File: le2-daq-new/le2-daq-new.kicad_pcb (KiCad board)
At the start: 2 copper layers, 62 x 105.9 mm, 9 parts, among them J1 RELAY-CONN, J2 CAP-CONN, J3 TC-CONN, J4 HX_CON, J5 Conn_01x02_Male, SW1 SW_Push, U1 ESP32-DEVKITC-32D

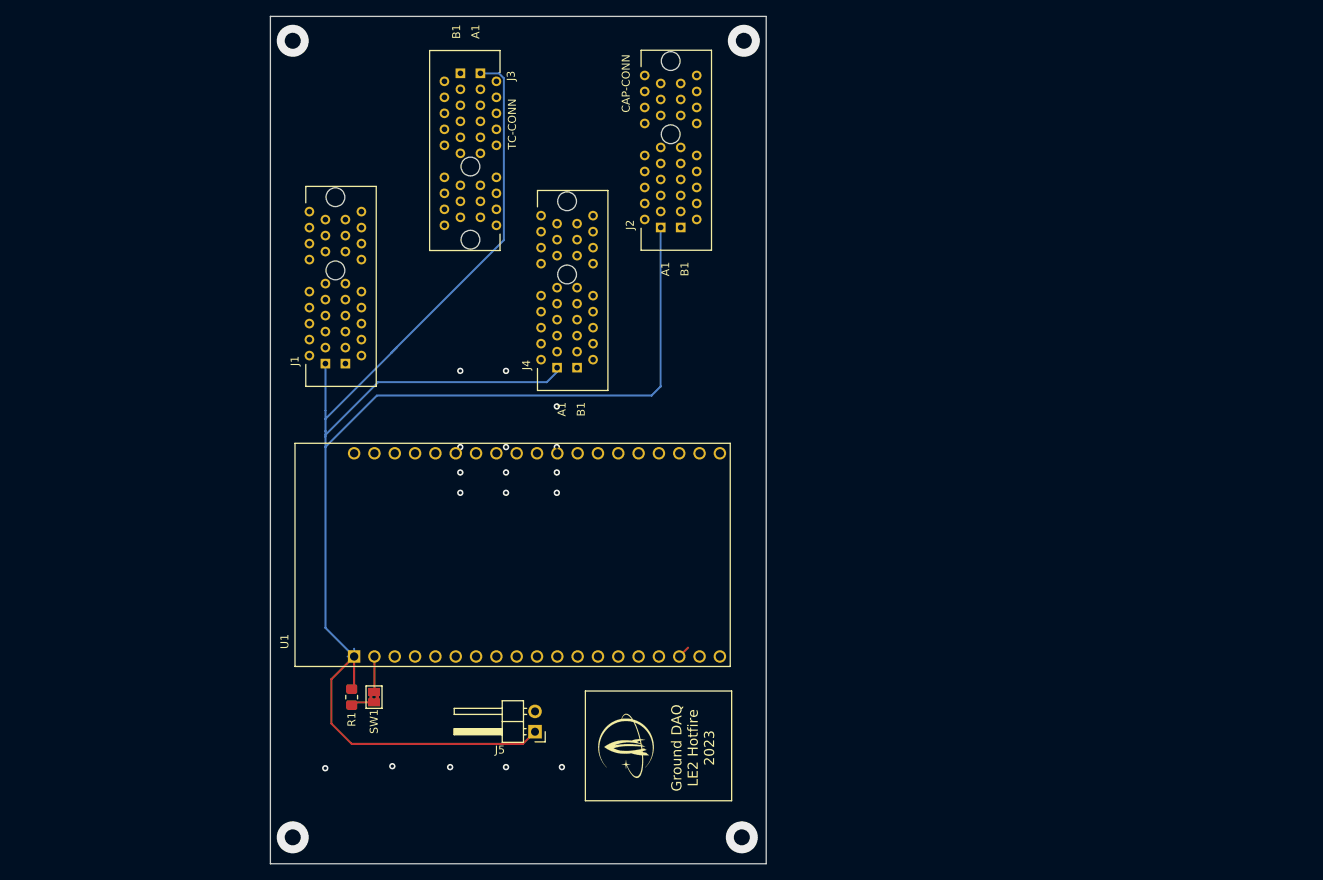
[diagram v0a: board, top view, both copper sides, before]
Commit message: CORE PCB DONE
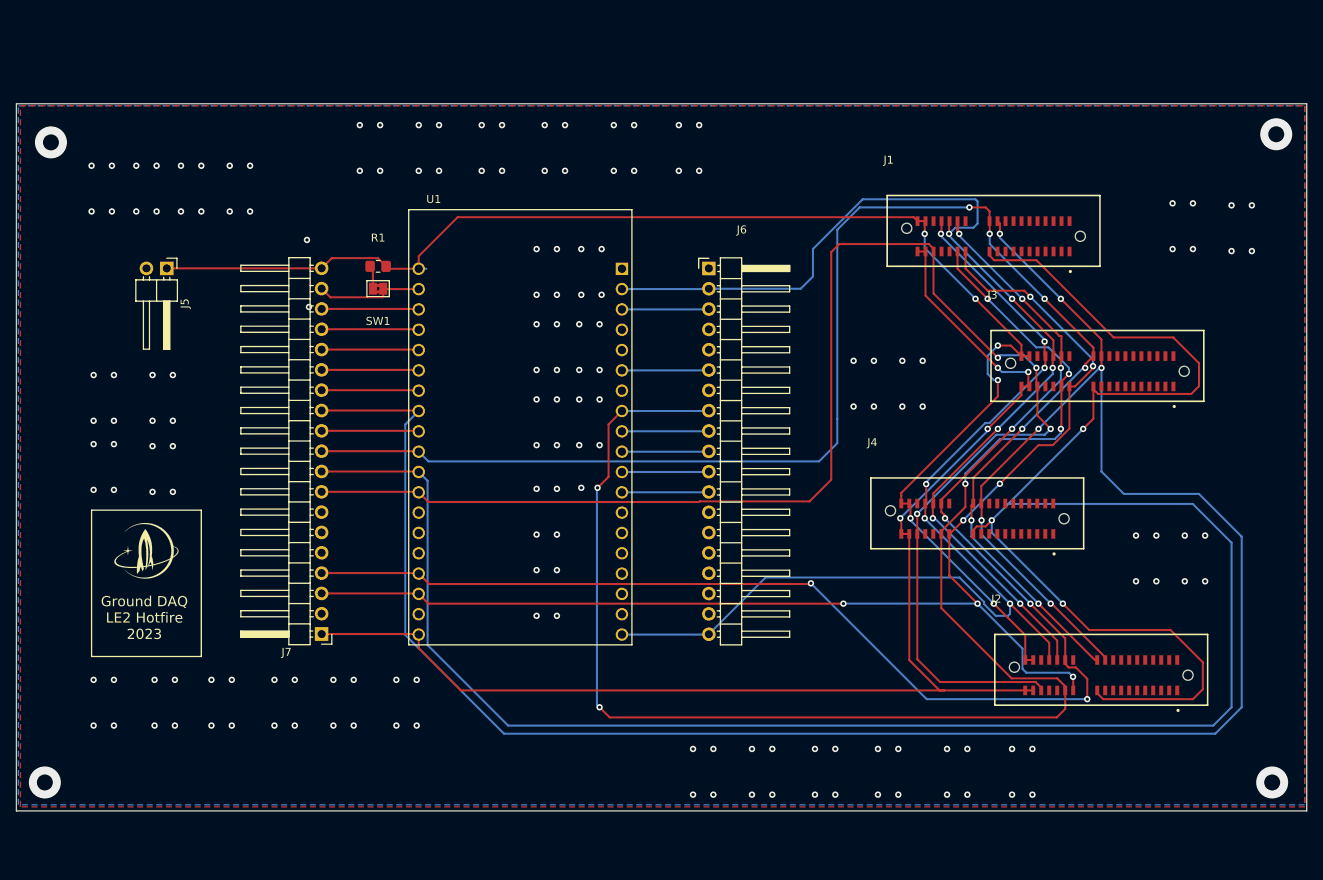
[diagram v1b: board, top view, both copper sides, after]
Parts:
- added J6: TEST-POINT, Connector_PinHeader_2.54mm:PinHeader_1x19_P2.54mm_Horizontal, F.Cu at (140.7, 78.2)
- added J7: TEST-POINT, Connector_PinHeader_2.54mm:PinHeader_1x19_P2.54mm_Horizontal, F.Cu at (92.3, 123.9)
- J1: value RELAY-CONN -> PCIE_CONN; footprint PCIE_1x_Socket:AMPHENOL_10018784-10210TLF -> PCIE-LP-01-01-F-DV-A-TR:SAMTEC_PCIE-LP-01-01-F-DV-A-TR
- J2: value CAP-CONN -> PCIE_CONN; footprint PCIE_1x_Socket:AMPHENOL_10018784-10210TLF -> PCIE-LP-01-01-F-DV-A-TR:SAMTEC_PCIE-LP-01-01-F-DV-A-TR
- J3: value TC-CONN -> PCIE_CONN; footprint PCIE_1x_Socket:AMPHENOL_10018784-10210TLF -> PCIE-LP-01-01-F-DV-A-TR:SAMTEC_PCIE-LP-01-01-F-DV-A-TR
- J4: value HX_CON -> PCIE_CONN; footprint PCIE_1x_Socket:AMPHENOL_10018784-10210TLF -> PCIE-LP-01-01-F-DV-A-TR:SAMTEC_PCIE-LP-01-01-F-DV-A-TR
- SW1: value SW_Push -> EN_HIGH
- moved J2 86.4 mm to (189.7, 129.1), turned to 0 degrees
- moved J3 82.4 mm to (189.2, 91.1), turned to 0 degrees
- moved J1 82.4 mm to (176.2, 74.2), turned to 0 degrees
- moved J5 74.0 mm to (72.9, 78.2), turned to -90 degrees
- moved G*** 64.7 mm to (70.4, 113.5), turned to 0 degrees
- moved J4 59.7 mm to (174.2, 109.5), turned to 0 degrees
- moved R1 53.9 mm to (99.3, 78.0), turned to 0 degrees
- moved SW1 51.1 mm to (99.3, 80.8), turned to 0 degrees
- moved U1 16.0 mm to (117.1, 98.0), turned to 0 degrees
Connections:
- net Net-(SW1-Pad2) renamed EN
- J1 pad A10: unconnected-(J1-PadA10) -> GND
- J1 pad A11: unconnected-(J1-PadA11) -> HX CLK
- J1 pad A12: unconnected-(J1-PadA12) -> CAP 2
- J1 pad A13: unconnected-(J1-PadA13) -> PHOTORES
- J1 pad A14: unconnected-(J1-PadA14) -> GND
- J1 pad A15: unconnected-(J1-PadA15) -> GND
- J1 pad A16: unconnected-(J1-PadA16) -> EXTRA
- J1 pad A17: unconnected-(J1-PadA17) -> +5V
- J1 pad A18: unconnected-(J1-PadA18) -> +5V
- J1 pad B10: unconnected-(J1-PadB10) -> HX 6
- J1 pad B11: unconnected-(J1-PadB11) -> HX 8
- J1 pad B12: unconnected-(J1-PadB12) -> GND
- J1 pad B13: unconnected-(J1-PadB13) -> CAP 1
- J1 pad B14: unconnected-(J1-PadB14) -> RL INT
- J1 pad B15: unconnected-(J1-PadB15) -> CAP CLK
- J1 pad B16: unconnected-(J1-PadB16) -> GND
- J1 pad B17: unconnected-(J1-PadB17) -> +3.3V
- J1 pad B18: unconnected-(J1-PadB18) -> +3.3V
- J2 pad A10: unconnected-(J2-PadA10) -> GND
- J2 pad A11: unconnected-(J2-PadA11) -> HX CLK
- J2 pad A12: unconnected-(J2-PadA12) -> CAP 2
- J2 pad A13: unconnected-(J2-PadA13) -> PHOTORES
- J2 pad A14: unconnected-(J2-PadA14) -> GND
- J2 pad A15: unconnected-(J2-PadA15) -> GND
- J2 pad A16: unconnected-(J2-PadA16) -> EXTRA
- J2 pad A17: unconnected-(J2-PadA17) -> +5V
- J2 pad A18: unconnected-(J2-PadA18) -> +5V
- J2 pad B10: unconnected-(J2-PadB10) -> HX 6
- J2 pad B11: unconnected-(J2-PadB11) -> HX 8
- J2 pad B12: unconnected-(J2-PadB12) -> GND
- J2 pad B13: unconnected-(J2-PadB13) -> CAP 1
- J2 pad B14: unconnected-(J2-PadB14) -> RL INT
- J2 pad B15: unconnected-(J2-PadB15) -> CAP CLK
- J2 pad B16: unconnected-(J2-PadB16) -> GND
- J2 pad B17: unconnected-(J2-PadB17) -> +3.3V
- J2 pad B18: unconnected-(J2-PadB18) -> +3.3V
- J3 pad A10: unconnected-(J3-PadA10) -> GND
- J3 pad A11: unconnected-(J3-PadA11) -> HX CLK
- J3 pad A12: unconnected-(J3-PadA12) -> CAP 2
- J3 pad A13: unconnected-(J3-PadA13) -> PHOTORES
- J3 pad A14: unconnected-(J3-PadA14) -> GND
- J3 pad A15: unconnected-(J3-PadA15) -> GND
- J3 pad A16: unconnected-(J3-PadA16) -> EXTRA
- J3 pad A17: unconnected-(J3-PadA17) -> +5V
- J3 pad A18: unconnected-(J3-PadA18) -> +5V
- J3 pad B10: unconnected-(J3-PadB10) -> HX 6
- J3 pad B11: unconnected-(J3-PadB11) -> HX 8
- J3 pad B12: unconnected-(J3-PadB12) -> GND
- J3 pad B13: unconnected-(J3-PadB13) -> CAP 1
- J3 pad B14: unconnected-(J3-PadB14) -> RL INT
- J3 pad B15: unconnected-(J3-PadB15) -> CAP CLK
- J3 pad B16: unconnected-(J3-PadB16) -> GND
- J3 pad B17: unconnected-(J3-PadB17) -> +3.3V
- J3 pad B18: unconnected-(J3-PadB18) -> +3.3V
- J4 pad A10: unconnected-(J4-PadA10) -> GND
- J4 pad A11: unconnected-(J4-PadA11) -> HX CLK
- J4 pad A12: unconnected-(J4-PadA12) -> CAP 2
- J4 pad A13: unconnected-(J4-PadA13) -> PHOTORES
- J4 pad A14: unconnected-(J4-PadA14) -> GND
- J4 pad A15: unconnected-(J4-PadA15) -> GND
- J4 pad A16: unconnected-(J4-PadA16) -> EXTRA
- J4 pad A17: unconnected-(J4-PadA17) -> +5V
- J4 pad A18: unconnected-(J4-PadA18) -> +5V
- J4 pad B10: unconnected-(J4-PadB10) -> HX 6
- J4 pad B11: unconnected-(J4-PadB11) -> HX 8
- J4 pad B12: unconnected-(J4-PadB12) -> GND
- J4 pad B13: unconnected-(J4-PadB13) -> CAP 1
- J4 pad B14: unconnected-(J4-PadB14) -> RL INT
- J4 pad B15: unconnected-(J4-PadB15) -> CAP CLK
- J4 pad B16: unconnected-(J4-PadB16) -> GND
- J4 pad B17: unconnected-(J4-PadB17) -> +3.3V
- J4 pad B18: unconnected-(J4-PadB18) -> +3.3V
- U1 pad 10: HXLC 1 -> HX 8
- U1 pad 11: HXLC 2 -> HX CLK
- U1 pad 12: HX CLK -> EXTRA
- U1 pad 19: unconnected-(U1-Pad19) -> +5V
- U1 pad 21: RL 1 -> RL INT
- U1 pad 22: RL 2 -> RL SCL
- U1 pad 25: RL 3 -> RL SDA
- U1 pad 27: RL 4 -> PHOTORES
- U1 pad 28: RL 5 -> TC2 CS
- U1 pad 29: RL 6 -> TC1 CS
- U1 pad 3: TC CLK -> HX 1
- U1 pad 30: RL 7 -> TC SDO
- U1 pad 31: RL 8 -> TC CLK
- U1 pad 35: CAP CLK -> unconnected-(U1-Pad35)
- U1 pad 38: unconnected-(U1-Pad38) -> CAP CLK
- U1 pad 4: TC SDO -> HX 2
- U1 pad 5: TC1 CS -> HX 3
- U1 pad 6: TC2 CS -> HX 4
- U1 pad 7: HXPT 1 -> HX 5
- U1 pad 8: HXPT 2 -> HX 6
- U1 pad 9: HXPT 3 -> HX 7
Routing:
- net HX CLK: track 0.00 -> 318.1 mm, vias 0 -> 3
- net HX 6: track 0.00 -> 280.2 mm, vias 0 -> 6
- net EXTRA: track 0.00 -> 194.8 mm, vias 0 -> 4
- net PHOTORES: track 0.00 -> 192.8 mm, vias 0 -> 6
- net HX 8: track 0.00 -> 187.6 mm, vias 0 -> 7
- net CAP 1: track 0.00 -> 182.5 mm, vias 0 -> 8
- net +5V: track 0.00 -> 166.5 mm, vias 0 -> 4
- net CAP 2: track 1.56 -> 165.1 mm, vias 0 -> 7
- net RL INT: track 0.00 -> 131.3 mm, vias 0 -> 6
- net CAP CLK: track 0.00 -> 128.4 mm, vias 0 -> 6
- net +3.3V: track 234.7 -> 181.6 mm, vias 0 -> 6
- net HX 7: track 0.00 -> 12.2 mm
- net HX 5: track 0.00 -> 12.2 mm
- net HX 4: track 0.00 -> 12.2 mm
- net HX 3: track 0.00 -> 12.2 mm
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- added copper zone on B.Cu, net (none)
- added copper zone on F.Cu, net GND
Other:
- board size 62 x 105.9 mm -> 161.3 x 88.4 mm
- board text removed: "CAP-CONN"
- board text removed: "TC-CONN"
